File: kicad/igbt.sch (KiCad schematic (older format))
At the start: 40 parts, among them J801 Screw_Terminal_01x15, J802 Screw_Terminal_01x15, U801 SI8660BD, U802 SI8662BD, U803 SN74LVC2G17DBVR, U804 SN74LVC2G17DBVR, U805 SN74LVC2G17DBVR, U806 SN74LVC2G17DBVR, U807 SN74LVC2G17DBVR, U808 SN74LVC2G17DBVR, U809 SN74LVC2G17DBVR, U810 SN74LVC2G17DBVR, U811 SN74LVC2G17DBVR, U812 SN74LVC2G17DBVR, U813 SI8660BD, U814 SI8662BD

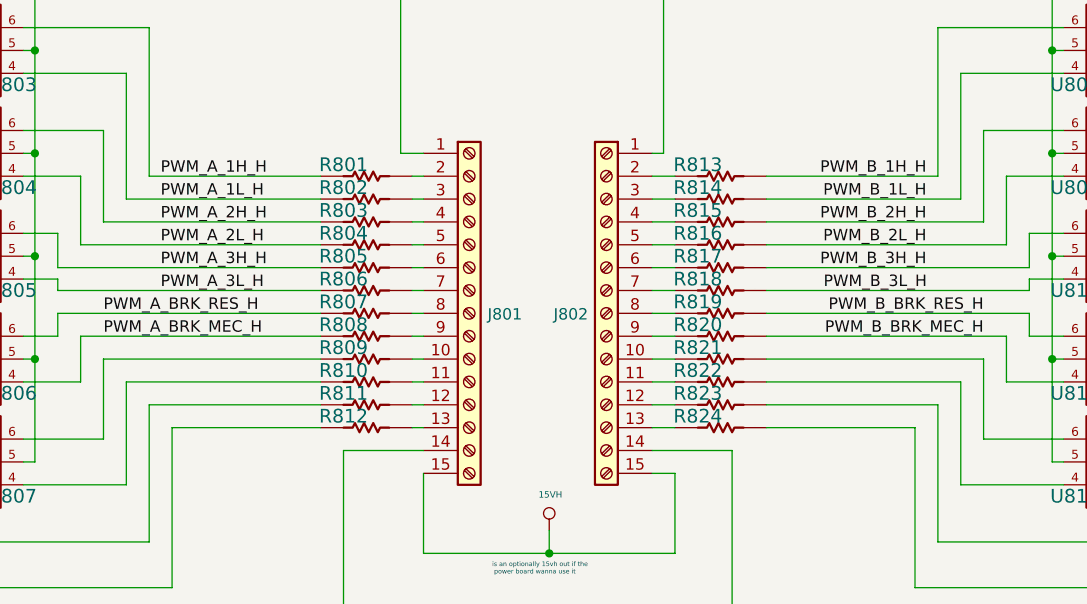
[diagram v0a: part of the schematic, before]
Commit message: begin PCB!! it's amess but IT IS
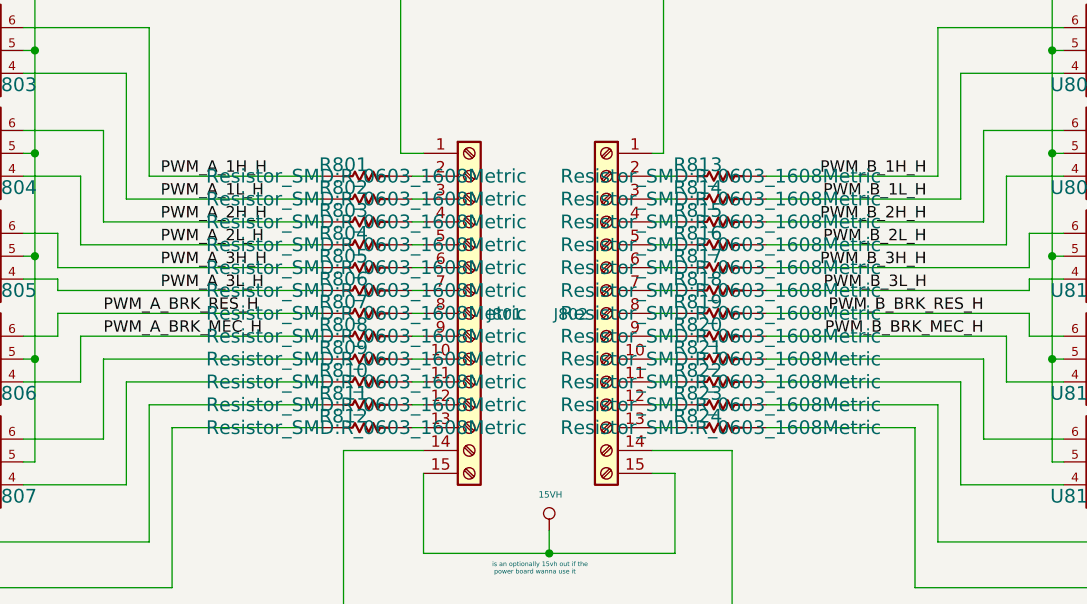
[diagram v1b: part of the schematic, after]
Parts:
- R801, R802, R803, R804, R805, R806, R807, R808, R809, R810, R811, R812, R813, R814, R815, R816, R817, R818, R819, R820, R821, R822, R823, R824: footprint (none) -> Resistor_SMD:R_0603_1608Metric
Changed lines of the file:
@@
 F 0 "R801" H 7200 3150 60  0000 C CNN
 F 1 "22e" H 7300 3203 60  0001 C CNN
-F 2 "" H 7300 3100 60  0000 C CNN
+F 2 "Resistor_SMD:R_0603_1608Metric" H 7300 3100 60  0000 C CNN
 F 3 "" H 7300 3100 60  0000 C CNN
 	1    7300 3100
@@
 F 0 "R802" H 7200 3250 60  0000 C CNN
 F 1 "22e" H 7300 3303 60  0001 C CNN
-F 2 "" H 7300 3200 60  0000 C CNN
+F 2 "Resistor_SMD:R_0603_1608Metric" H 7300 3200 60  0000 C CNN
 F 3 "" H 7300 3200 60  0000 C CNN
 	1    7300 3200
@@
 F 0 "R803" H 7200 3350 60  0000 C CNN
 F 1 "22e" H 7300 3403 60  0001 C CNN
-F 2 "" H 7300 3300 60  0000 C CNN
+F 2 "Resistor_SMD:R_0603_1608Metric" H 7300 3300 60  0000 C CNN
 F 3 "" H 7300 3300 60  0000 C CNN
 	1    7300 3300
@@
 F 0 "R804" H 7200 3450 60  0000 C CNN
 F 1 "22e" H 7300 3503 60  0001 C CNN
-F 2 "" H 7300 3400 60  0000 C CNN
+F 2 "Resistor_SMD:R_0603_1608Metric" H 7300 3400 60  0000 C CNN
 F 3 "" H 7300 3400 60  0000 C CNN
 	1    7300 3400
@@
 F 0 "R805" H 7200 3550 60  0000 C CNN
 F 1 "22e" H 7300 3603 60  0001 C CNN
-F 2 "" H 7300 3500 60  0000 C CNN
+F 2 "Resistor_SMD:R_0603_1608Metric" H 7300 3500 60  0000 C CNN
 F 3 "" H 7300 3500 60  0000 C CNN
 	1    7300 3500
@@
 F 0 "R806" H 7200 3650 60  0000 C CNN
 F 1 "22e" H 7300 3703 60  0001 C CNN
-F 2 "" H 7300 3600 60  0000 C CNN
+F 2 "Resistor_SMD:R_0603_1608Metric" H 7300 3600 60  0000 C CNN
 F 3 "" H 7300 3600 60  0000 C CNN
 	1    7300 3600
@@
 F 0 "R807" H 7200 3750 60  0000 C CNN
 F 1 "22e" H 7300 3803 60  0001 C CNN
-F 2 "" H 7300 3700 60  0000 C CNN
+F 2 "Resistor_SMD:R_0603_1608Metric" H 7300 3700 60  0000 C CNN
 F 3 "" H 7300 3700 60  0000 C CNN
 	1    7300 3700
@@
 F 0 "R808" H 7200 3850 60  0000 C CNN
 F 1 "22e" H 7300 3903 60  0001 C CNN
-F 2 "" H 7300 3800 60  0000 C CNN
+F 2 "Resistor_SMD:R_0603_1608Metric" H 7300 3800 60  0000 C CNN
 F 3 "" H 7300 3800 60  0000 C CNN
 	1    7300 3800
@@
 F 0 "R809" H 7200 3950 60  0000 C CNN
 F 1 "22e" H 7300 4003 60  0001 C CNN
-F 2 "" H 7300 3900 60  0000 C CNN
+F 2 "Resistor_SMD:R_0603_1608Metric" H 7300 3900 60  0000 C CNN
 F 3 "" H 7300 3900 60  0000 C CNN
 	1    7300 3900
@@
 F 0 "R810" H 7200 4050 60  0000 C CNN
 F 1 "22e" H 7300 4103 60  0001 C CNN
-F 2 "" H 7300 4000 60  0000 C CNN
+F 2 "Resistor_SMD:R_0603_1608Metric" H 7300 4000 60  0000 C CNN
 F 3 "" H 7300 4000 60  0000 C CNN
 	1    7300 4000
@@
 F 0 "R811" H 7200 4150 60  0000 C CNN
 F 1 "22e" H 7300 4203 60  0001 C CNN
-F 2 "" H 7300 4100 60  0000 C CNN
+F 2 "Resistor_SMD:R_0603_1608Metric" H 7300 4100 60  0000 C CNN
 F 3 "" H 7300 4100 60  0000 C CNN
 	1    7300 4100
@@
 F 0 "R812" H 7200 4250 60  0000 C CNN
 F 1 "22e" H 7300 4303 60  0001 C CNN
-F 2 "" H 7300 4200 60  0000 C CNN
+F 2 "Resistor_SMD:R_0603_1608Metric" H 7300 4200 60  0000 C CNN
 F 3 "" H 7300 4200 60  0000 C CNN
 	1    7300 4200
@@
 F 0 "R813" H 8750 3150 60  0000 C CNN
 F 1 "22e" H 8850 3203 60  0001 C CNN
-F 2 "" H 8850 3100 60  0000 C CNN
+F 2 "Resistor_SMD:R_0603_1608Metric" H 8850 3100 60  0000 C CNN
 F 3 "" H 8850 3100 60  0000 C CNN
 	1    8850 3100
@@
 F 0 "R814" H 8750 3250 60  0000 C CNN
 F 1 "22e" H 8850 3303 60  0001 C CNN
-F 2 "" H 8850 3200 60  0000 C CNN
+F 2 "Resistor_SMD:R_0603_1608Metric" H 8850 3200 60  0000 C CNN
 F 3 "" H 8850 3200 60  0000 C CNN
 	1    8850 3200
@@
 F 0 "R815" H 8750 3350 60  0000 C CNN
 F 1 "22e" H 8850 3403 60  0001 C CNN
-F 2 "" H 8850 3300 60  0000 C CNN
+F 2 "Resistor_SMD:R_0603_1608Metric" H 8850 3300 60  0000 C CNN
 F 3 "" H 8850 3300 60  0000 C CNN
 	1    8850 3300
@@
 F 0 "R816" H 8750 3450 60  0000 C CNN
 F 1 "22e" H 8850 3503 60  0001 C CNN
-F 2 "" H 8850 3400 60  0000 C CNN
+F 2 "Resistor_SMD:R_0603_1608Metric" H 8850 3400 60  0000 C CNN
 F 3 "" H 8850 3400 60  0000 C CNN
 	1    8850 3400
@@
 F 0 "R817" H 8750 3550 60  0000 C CNN
 F 1 "22e" H 8850 3603 60  0001 C CNN
-F 2 "" H 8850 3500 60  0000 C CNN
+F 2 "Resistor_SMD:R_0603_1608Metric" H 8850 3500 60  0000 C CNN
 F 3 "" H 8850 3500 60  0000 C CNN
 	1    8850 3500
@@
 F 0 "R818" H 8750 3650 60  0000 C CNN
 F 1 "22e" H 8850 3703 60  0001 C CNN
-F 2 "" H 8850 3600 60  0000 C CNN
+F 2 "Resistor_SMD:R_0603_1608Metric" H 8850 3600 60  0000 C CNN
 F 3 "" H 8850 3600 60  0000 C CNN
 	1    8850 3600
@@
 F 0 "R819" H 8750 3750 60  0000 C CNN
 F 1 "22e" H 8850 3803 60  0001 C CNN
-F 2 "" H 8850 3700 60  0000 C CNN
+F 2 "Resistor_SMD:R_0603_1608Metric" H 8850 3700 60  0000 C CNN
 F 3 "" H 8850 3700 60  0000 C CNN
 	1    8850 3700
@@
 F 0 "R820" H 8750 3850 60  0000 C CNN
 F 1 "22e" H 8850 3903 60  0001 C CNN
-F 2 "" H 8850 3800 60  0000 C CNN
+F 2 "Resistor_SMD:R_0603_1608Metric" H 8850 3800 60  0000 C CNN
 F 3 "" H 8850 3800 60  0000 C CNN
 	1    8850 3800
@@
 F 0 "R821" H 8750 3950 60  0000 C CNN
 F 1 "22e" H 8850 4003 60  0001 C CNN
-F 2 "" H 8850 3900 60  0000 C CNN
+F 2 "Resistor_SMD:R_0603_1608Metric" H 8850 3900 60  0000 C CNN
 F 3 "" H 8850 3900 60  0000 C CNN
 	1    8850 3900
@@
 F 0 "R822" H 8750 4050 60  0000 C CNN
 F 1 "22e" H 8850 4103 60  0001 C CNN
-F 2 "" H 8850 4000 60  0000 C CNN
+F 2 "Resistor_SMD:R_0603_1608Metric" H 8850 4000 60  0000 C CNN
 F 3 "" H 8850 4000 60  0000 C CNN
 	1    8850 4000
@@
 F 0 "R823" H 8750 4150 60  0000 C CNN
 F 1 "22e" H 8850 4203 60  0001 C CNN
-F 2 "" H 8850 4100 60  0000 C CNN
+F 2 "Resistor_SMD:R_0603_1608Metric" H 8850 4100 60  0000 C CNN
 F 3 "" H 8850 4100 60  0000 C CNN
 	1    8850 4100
@@
 F 0 "R824" H 8750 4250 60  0000 C CNN
 F 1 "22e" H 8850 4303 60  0001 C CNN
-F 2 "" H 8850 4200 60  0000 C CNN
+F 2 "Resistor_SMD:R_0603_1608Metric" H 8850 4200 60  0000 C CNN
 F 3 "" H 8850 4200 60  0000 C CNN
 	1    8850 4200

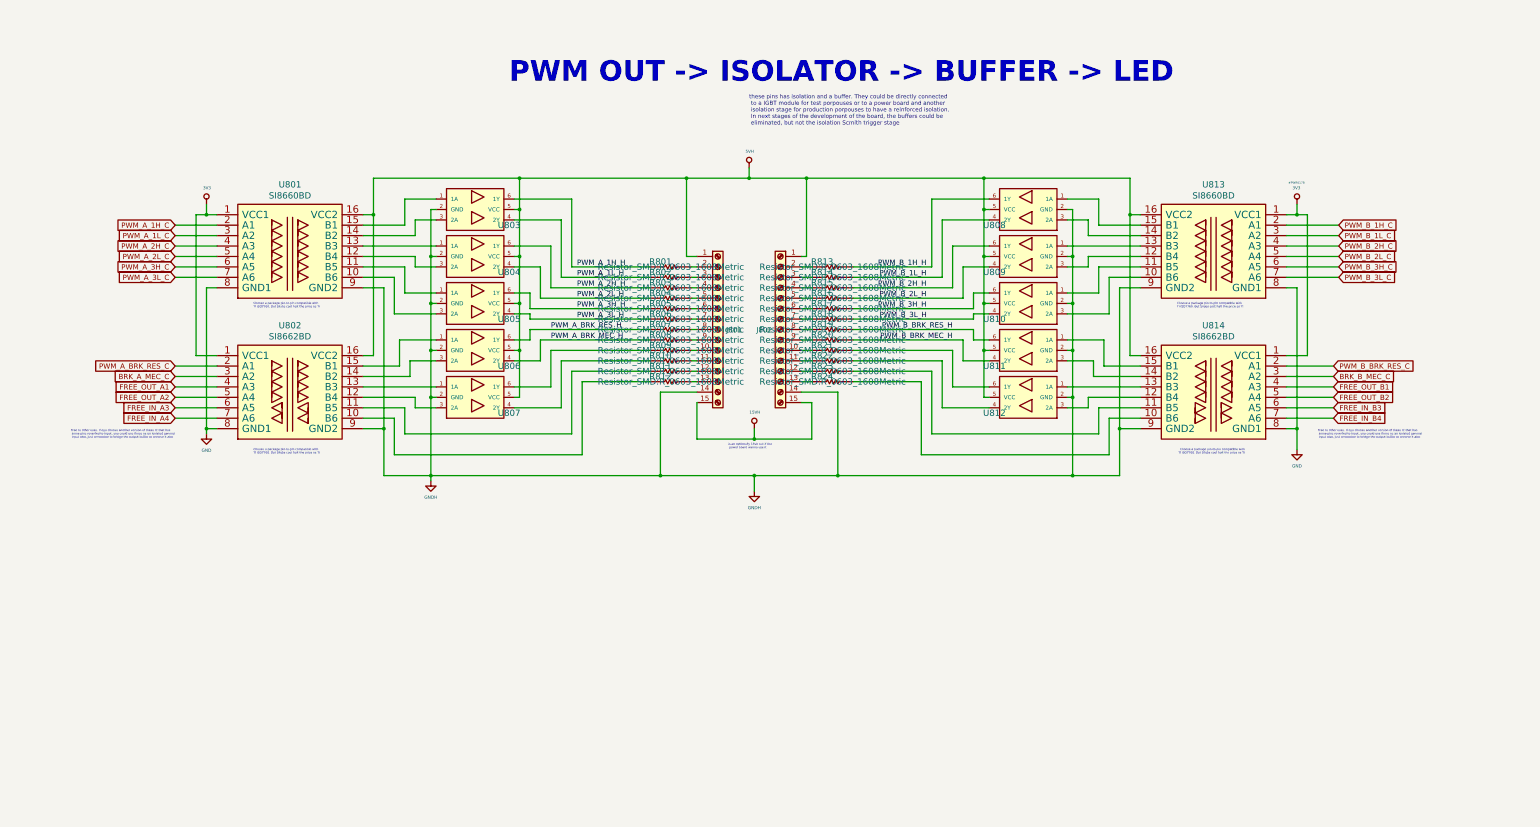
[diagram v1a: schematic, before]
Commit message: I've passed all footprin to layout BUT...
I've passed all, first glance... I need to confirm in details a lot of
things. The objetive for these is to have an aproximation of the size
I'll need to make the board.. then I choose the final detailed footprint
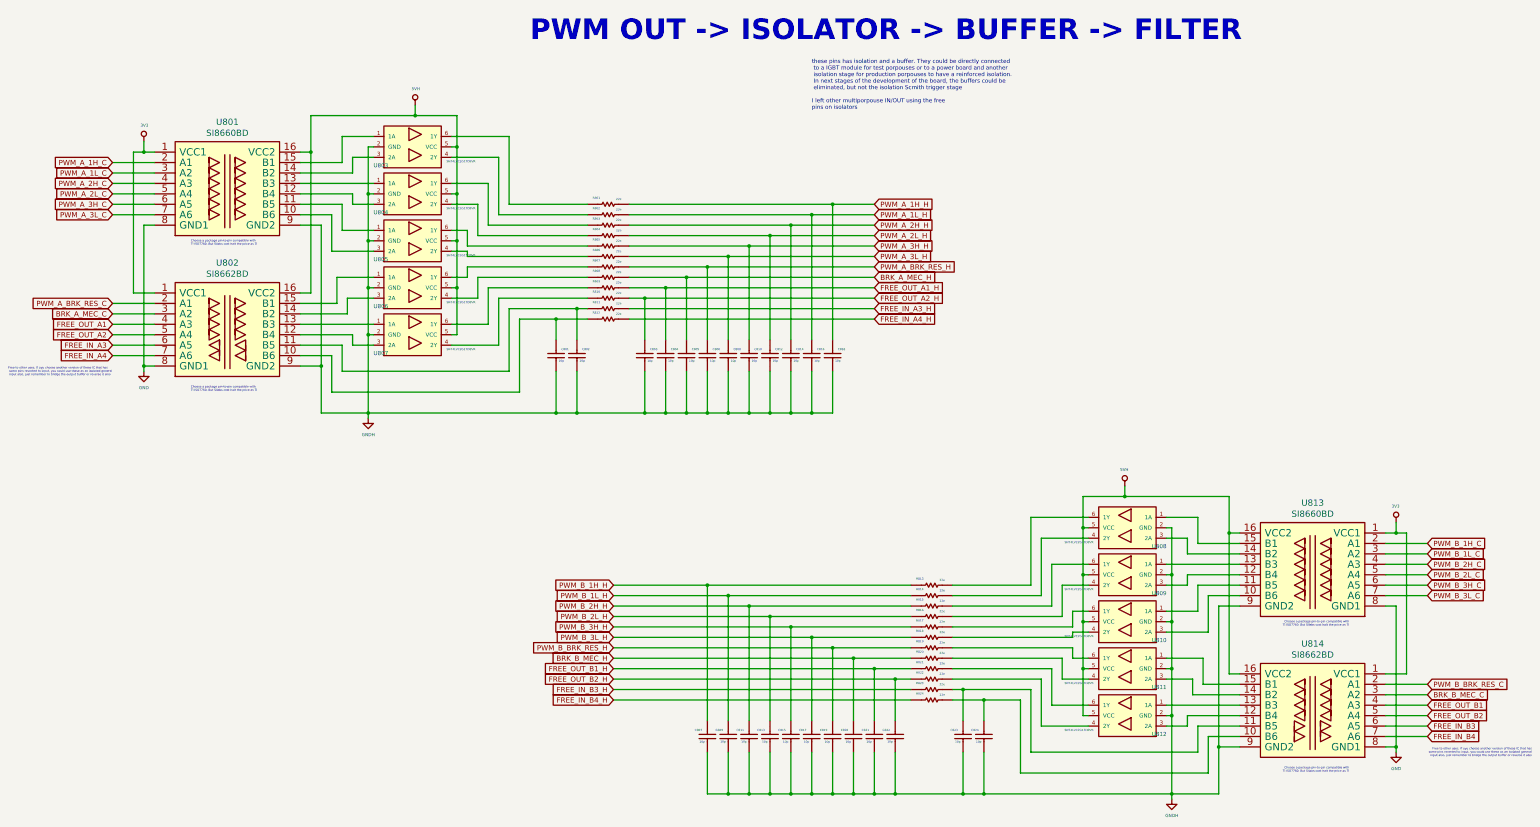
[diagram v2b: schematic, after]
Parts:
- removed J801, J802: Screw_Terminal_01x15, symbol Connector:Screw_Terminal_01x15
- added C801, C802, C803, C804, C805, C806, C807, C808, C809, C810, C811, C812, C813, C814, C815, C816, C817, C818, C819, C820, C821, C822, C823, C824: 10p, servo:C_0603_1608Metric, symbol servo:Capacitor
- U801, U802, U813, U814: footprint (none) -> Package_SO:SOIC-16W_7.5x10.3mm_P1.27mm
- U803, U804, U805, U806, U807, U808, U809, U810, U811, U812: footprint (none) -> servo:SOT-23-6
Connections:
- net GNDH: now also C801.1, C802.1, C803.1, C804.1, C805.1, C806.1, C807.1, C808.1, C809.1, C810.1, C811.1, C812.1, C813.1, C814.1, C815.1, C816.1, C817.1, C818.1, C819.1, C820.1, C821.1, C822.1, C823.1, C824.1
- net PWM_A_1H_H: now also R801.2, C818.2 (Capacitor); no longer R801.1, U803.6 (1Y)
- net PWM_A_1L_H: now also R802.2, C816.2 (Capacitor); no longer R802.1, U803.4 (2Y)
- net PWM_A_2H_H: now also R803.2, C814.2 (Capacitor); no longer R803.1, U804.6 (1Y)
- net PWM_A_2L_H: now also R804.2, C812.2 (Capacitor); no longer R804.1, U804.4 (2Y)
- net PWM_A_3H_H: now also R805.2, C810.2 (Capacitor); no longer R805.1, U805.6 (1Y)
- net PWM_A_3L_H: now also R806.2, C808.2 (Capacitor); no longer R806.1, U805.4 (2Y)
- net PWM_A_BRK_RES_H: now also R807.2, C806.2 (Capacitor); no longer R807.1, U806.6 (1Y)
- net PWM_B_1H_H: now also R813.1, C807.2 (Capacitor); no longer R813.2, U808.6 (1Y)
- net PWM_B_1L_H: now also R814.1, C809.2 (Capacitor); no longer R814.2, U808.4 (2Y)
- net PWM_B_2H_H: now also R815.1, C811.2 (Capacitor); no longer R815.2, U809.6 (1Y)
- net PWM_B_2L_H: now also R816.1, C813.2 (Capacitor); no longer R816.2, U809.4 (2Y)
- net PWM_B_3H_H: now also R817.1, C815.2 (Capacitor); no longer R817.2, U810.6 (1Y)
- net PWM_B_3L_H: now also R818.1, C817.2 (Capacitor); no longer R818.2, U810.4 (2Y)
- net PWM_B_BRK_RES_H: now also R819.1, C819.2 (Capacitor); no longer R819.2, U811.6 (1Y)
- net BRK_A_MEC_H: now reaches R808.2
- net BRK_A_MEC_H: now also C805.2 (Capacitor)
- net FREE_OUT_A1_H: now reaches R809.2
- net FREE_OUT_A1_H: now also C804.2 (Capacitor)
- net FREE_OUT_A2_H: now reaches R810.2
- net FREE_OUT_A2_H: now also C803.2 (Capacitor)
- net at R811.1, U802.11 (B5): now also C802.2 (Capacitor)
- net FREE_IN_A3_H: now reaches R811.2
- net at R812.1, U802.10 (B6): now also C801.2 (Capacitor)
- net FREE_IN_A4_H: now reaches R812.2
- net BRK_B_MEC_H: now reaches R820.1
- net BRK_B_MEC_H: now also C820.2 (Capacitor)
- net FREE_OUT_B1_H: now reaches R821.1
- net FREE_OUT_B1_H: now also C821.2 (Capacitor)
- net FREE_OUT_B2_H: now reaches R822.1
- net FREE_OUT_B2_H: now also C822.2 (Capacitor)
- net FREE_IN_B3_H: now reaches R823.1
- net at R823.2, U814.11 (B5): now also C823.2 (Capacitor)
- net FREE_IN_B4_H: now reaches R824.1
- net at R824.2, U814.10 (B6): now also C824.2 (Capacitor)
- net PWM_A_BRK_MEC_H: no longer names the net of R808.1, U806.4 (2Y)
- net PWM_B_BRK_MEC_H: no longer names the net of R820.2, U811.4 (2Y)
- new net: R807.1, U806.6 (1Y)
- new net: R806.1, U805.4 (2Y)
- new net: R805.1, U805.6 (1Y)
- new net: R804.1, U804.4 (2Y)
- new net: R803.1, U804.6 (1Y)
- new net: R802.1, U803.4 (2Y)
- new net: R801.1, U803.6 (1Y)
- new net: R819.2, U811.6 (1Y)
- new net: R818.2, U810.4 (2Y)
- new net: R817.2, U810.6 (1Y)
- new net: R816.2, U809.4 (2Y)
- new net: R815.2, U809.6 (1Y)
- new net: R814.2, U808.4 (2Y)
- new net: R813.2, U808.6 (1Y)
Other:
- note added: "PWM OUT -> ISOLATOR -> BUFFER -> FILTER\n"
- note added: "these pins has isolation and a buffer. They could be directly connected\n to a IGBT module for test porpouses or to a power board and another\n isolation stage for production porpouses to have a reinforced isolation.\n In next stages of the development of the board, the buffers could be\n eliminated, but not the isolation Scmith trigger stage\n\nI left other multiporpouse IN/OUT using the free \n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"
- note removed: "PWM OUT -> ISOLATOR -> BUFFER -> LED"
- note removed: "is an optionally 15vh out if the\n power board wanna use it"
- note removed: "these pins has isolation and a buffer. They could be directly connected\n to a IGBT module for test porpouses or to a power board and another\n isolation stage for production porpouses to have a reinforced isolation.\n In next stages of the development of the board, the buffers could be\n eliminated, but not the isolation Scmith trigger stage"
